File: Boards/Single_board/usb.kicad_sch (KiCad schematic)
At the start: 2 parts, among them J3 USB_C_Receptacle_USB2.0_16P, U3 CH340G

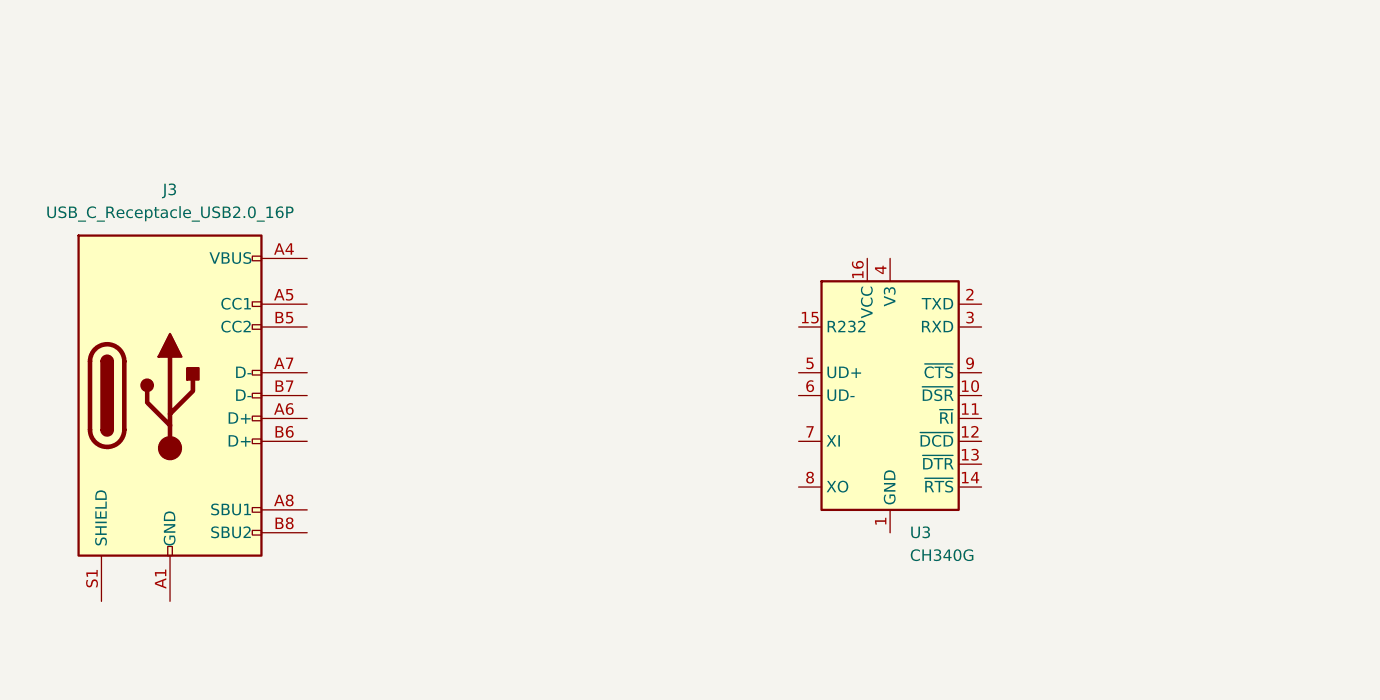
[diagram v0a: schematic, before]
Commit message: Single board nearly ready to order
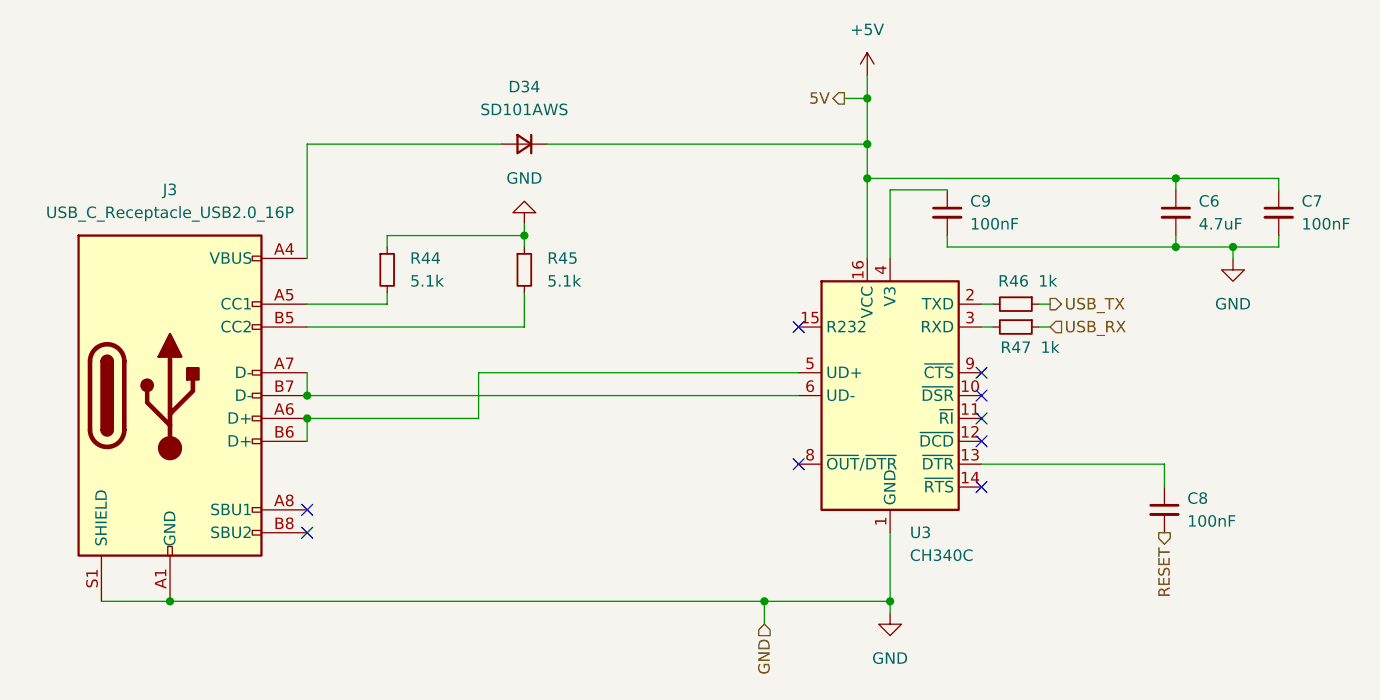
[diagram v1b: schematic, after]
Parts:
- removed U3: CH340G, Package_SO:SOIC-16_3.9x9.9mm_P1.27mm, symbol Interface_USB:CH340G
- added C6: 4.7uF, Capacitor_SMD:C_0805_2012Metric, symbol Device:C_Small
- added C7, C8, C9: 100nF, Capacitor_SMD:C_0805_2012Metric, symbol Device:C_Small
- added D34: SD101AWS, Diode_SMD:D_SOD-323, symbol Device:D_Small
- added R44, R45: 5.1k, Resistor_SMD:R_0603_1608Metric, symbol Device:R_Small
- added R46, R47: 1k, Resistor_SMD:R_0603_1608Metric, symbol Device:R_Small
- added U3: CH340C, Package_SO:SOIC-16_3.9x9.9mm_P1.27mm, symbol Interface_USB:CH340C
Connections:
- net GND: now reaches J3.A1 (GND), J3.A12 (GND), J3.B1 (GND), J3.B12 (GND)
- net GND: now also J3.S1 (SHIELD), C6.2, C7.2, C9.2, R44.1, R45.1, U3.1 (GND)
- net at J3.A4 (VBUS), J3.A9 (VBUS), J3.B4 (VBUS)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: now also D34.2 (A)
- net at J3.A5 (CC1): now also R44.2
- net at J3.A6 (D+): now also J3.B6 (D+), U3.5 (UD+)
- net at J3.A7 (D-): now also J3.B7 (D-), U3.6 (UD-)
- net at J3.B5 (CC2): now also R45.2
- new net: C9.1, U3.4 (V3)
- new net: R46.2, U3.2 (TXD)
- new net: C8.1, U3.13 (~{DTR})
- new net: R47.2, U3.3 (RXD)
- new net +5V: C6.1, C7.1, D34.1 (K), U3.16 (VCC)
- new net RESET: C8.2
- new net USB_RX: R47.1
- new net USB_TX: R46.1
- no-connect marks 0 -> 9
